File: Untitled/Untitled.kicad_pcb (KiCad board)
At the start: 2 copper layers, 31 parts, among them SW1 MX_SW_HS, SW2 MX_SW_HS, SW4 RST, SW6 MX_SW_HS, SW7 MX_SW_HS, SW8 MX_SW_HS, SW9 MX_SW_HS, U1 nice_nano

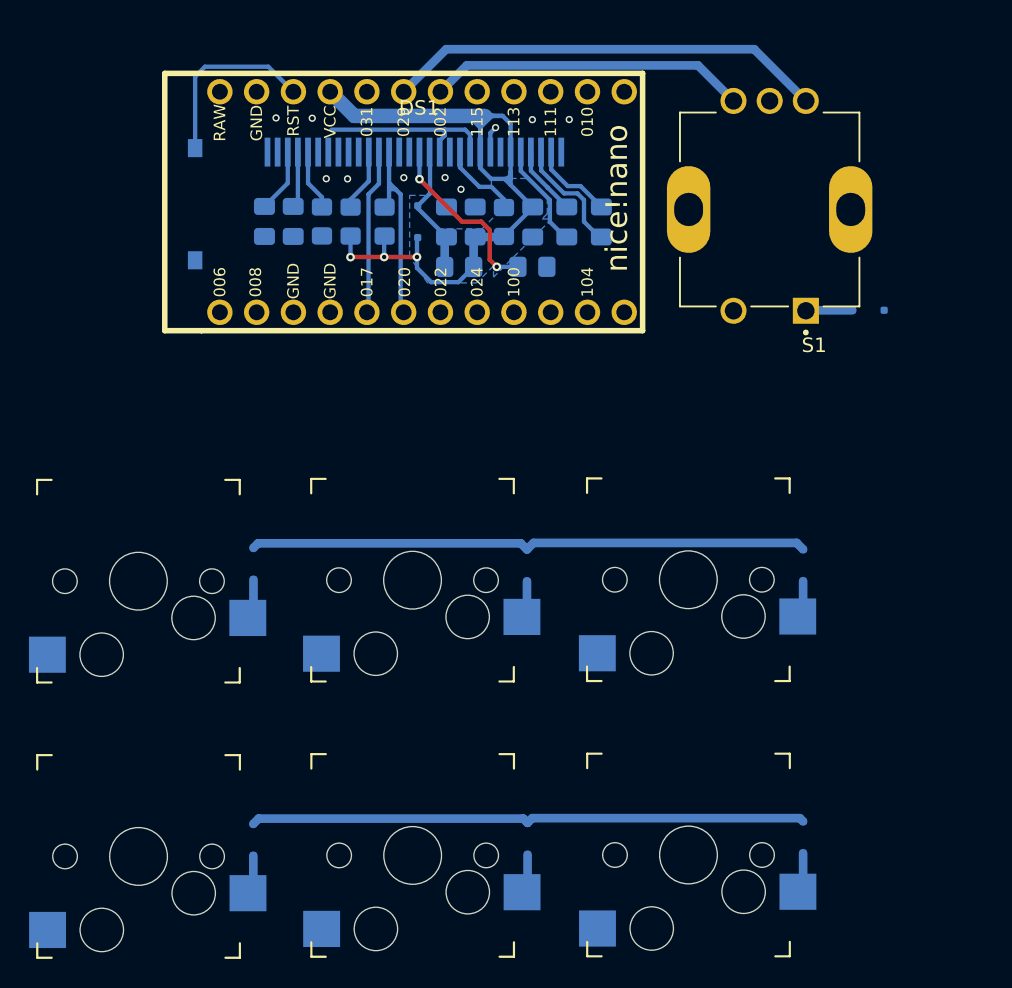
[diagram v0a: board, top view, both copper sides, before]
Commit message: idk
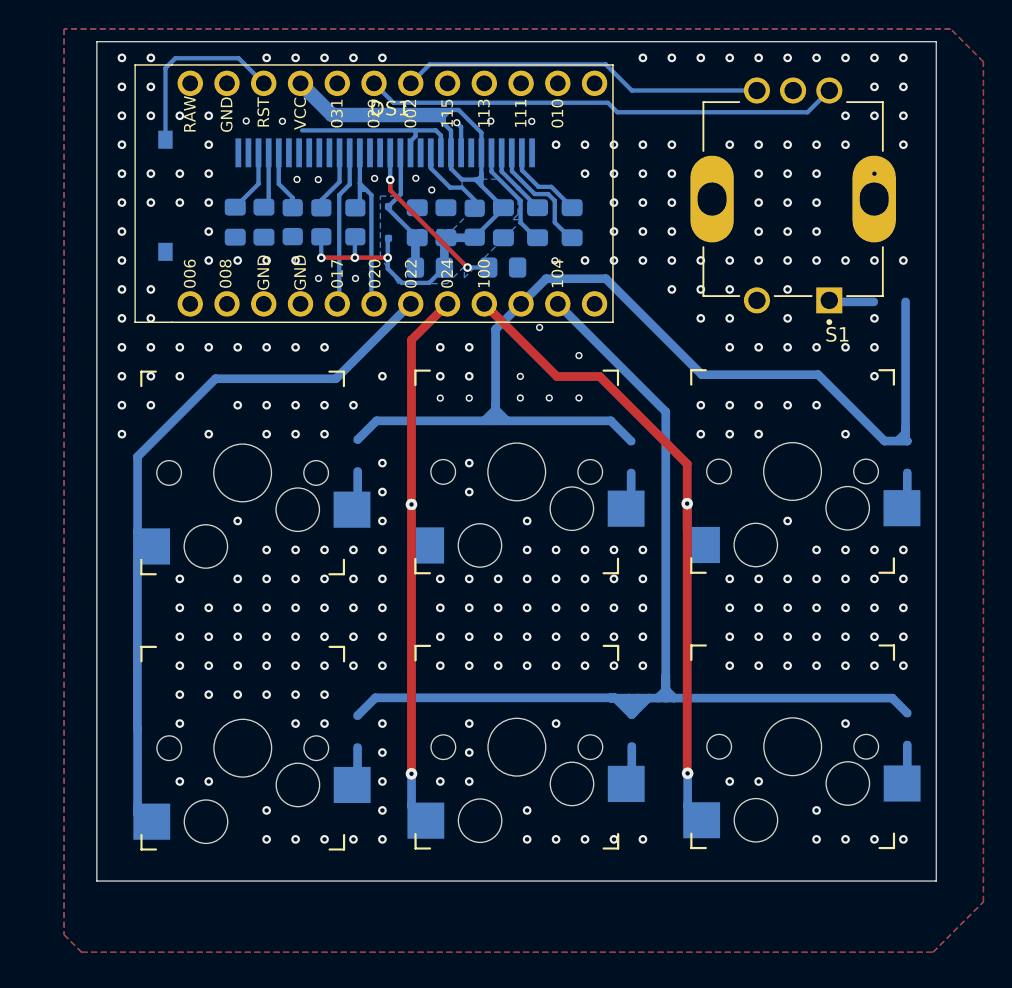
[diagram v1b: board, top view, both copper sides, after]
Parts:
- moved D3 10.4 mm to (152.7, 72.3)
- moved D4 10.4 mm to (171.6, 72.4)
- moved D6 10.4 mm to (171.6, 91.3)
- moved SW2 10.4 mm to (182.7, 92.5)
- moved SW8 10.4 mm to (144.7, 92.5)
- moved SW9 10.4 mm to (163.7, 92.5)
- moved SW6 10.4 mm to (144.7, 73.5)
- moved SW7 10.4 mm to (163.7, 73.5)
- moved D2 10.4 mm to (190.7, 72.4)
- moved D5 10.4 mm to (152.7, 91.4)
- moved D7 10.4 mm to (190.7, 91.2)
- moved SW1 10.4 mm to (182.7, 73.4)
- moved SW4 2.13 mm to (139.4, 54.4)
- moved U1 2.13 mm to (155.1, 54.2)
- moved C2 2.02 mm to (158.8, 56.2)
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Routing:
- net col0: track 0.00 -> 49.9 mm
- net col2: track 0.00 -> 46.9 mm, vias 0 -> 2
- net col1: track 0.00 -> 40.4 mm, vias 0 -> 2
- net row1: track 38.5 -> 78.1 mm
- net row0: track 38.7 -> 73.4 mm
- net +3.3V: track 52.4 -> 49.0 mm
- net ROT2: track 22.0 -> 25.2 mm
- net ROT1: track 30.5 -> 32.9 mm
- net Net-(DS1-D/~{C}): track 12.4 -> 11.6 mm
- net GND: track 14.5 -> 14.8 mm, vias 10 -> 327
- added copper zone on B.Cu, net GND
- added copper zone on F.Cu, net GND
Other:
- board outline added: 58 x 58 mm
